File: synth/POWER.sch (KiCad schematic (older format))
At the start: 13 parts, among them J1 9V_BAT_HOLDER, SW2 SW_SPDT, U3 SCD7805BTG

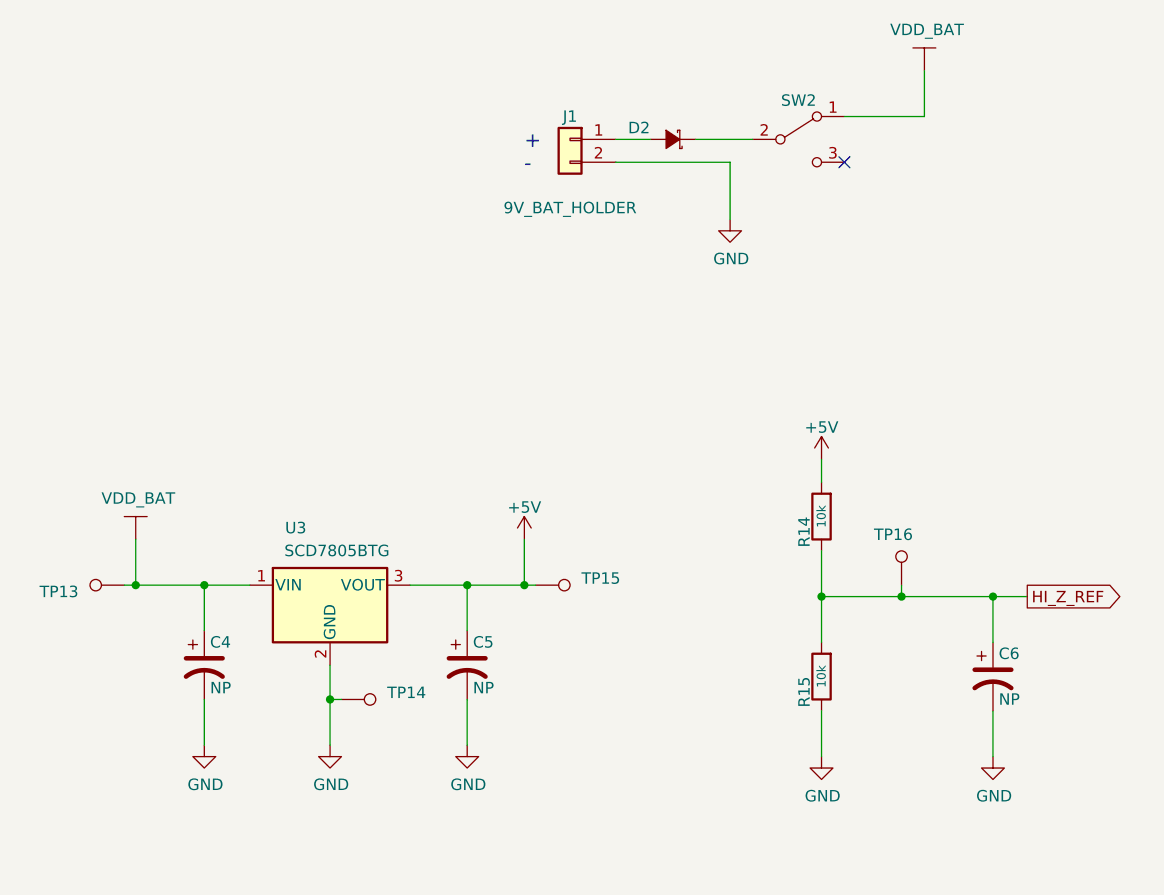
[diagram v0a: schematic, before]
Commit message: automated commit
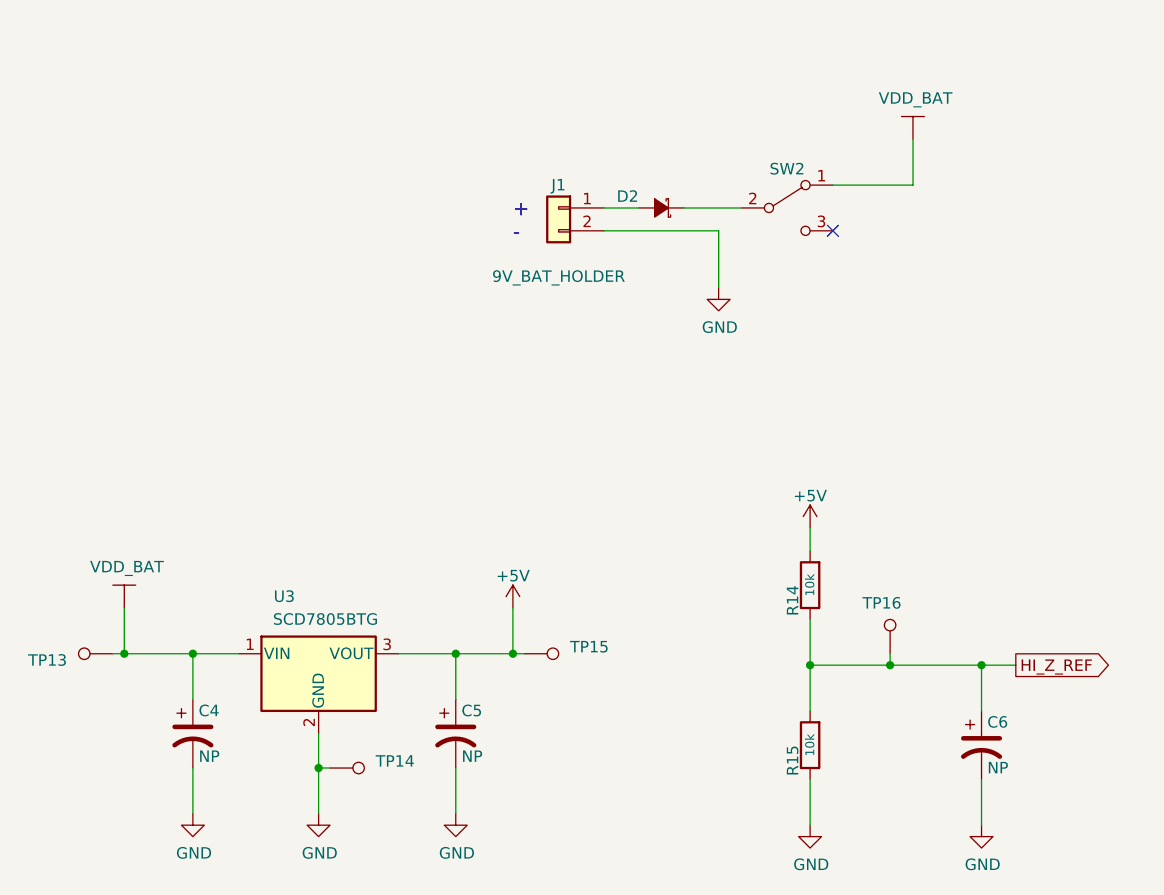
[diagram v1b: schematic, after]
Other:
- moved on the sheet: C4, C5, C6, D2, J1, R14, R15, SW2, TP13, TP14, TP15, TP16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
